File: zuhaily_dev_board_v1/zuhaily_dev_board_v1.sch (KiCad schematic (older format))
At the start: 43 parts

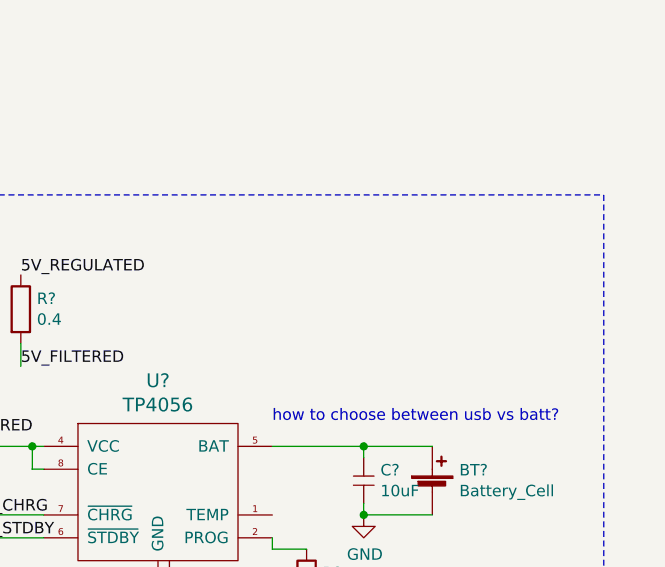
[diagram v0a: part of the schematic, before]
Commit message: branch commit
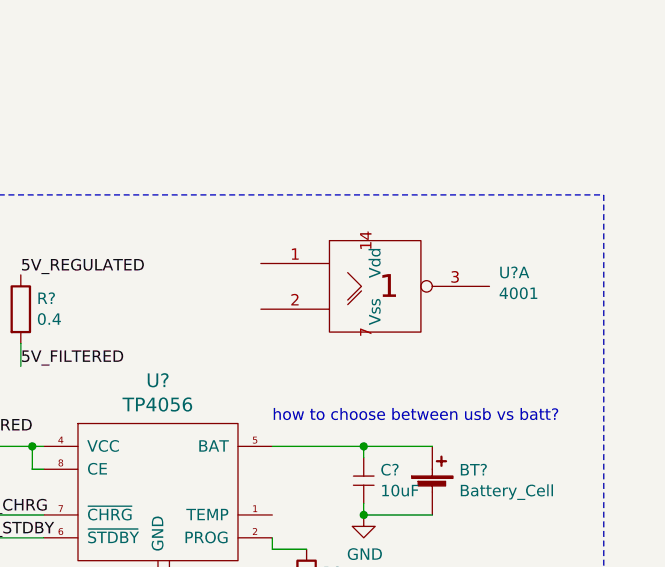
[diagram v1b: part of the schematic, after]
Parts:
- added U?: 4001, symbol 4xxx_IEEE:4001
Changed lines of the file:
@@
+	1    0    0    -1
+$EndComp
+$Comp
+L 4xxx_IEEE:4001 U?
+U 1 1 5C5155E3
+P 17750 2550
+F 0 "U?" H 18291 2609 50  0000 L CNN
+F 1 "4001" H 18291 2518 50  0000 L CNN
+F 2 "" H 17750 2550 50  0001 C CNN
+F 3 "" H 17750 2550 50  0001 C CNN
+	1    17750 2550
 	1    0    0    -1
 $EndComp
